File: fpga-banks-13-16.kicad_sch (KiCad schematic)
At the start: 40 parts, among them U14 XC7A100T-FGG484, U15 Oscillator_100MHz_AMJMEFB

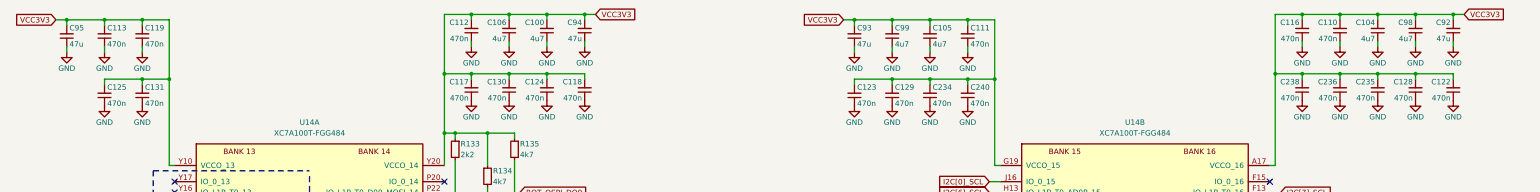
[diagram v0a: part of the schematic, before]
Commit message: [#82378] Project refresh 81589
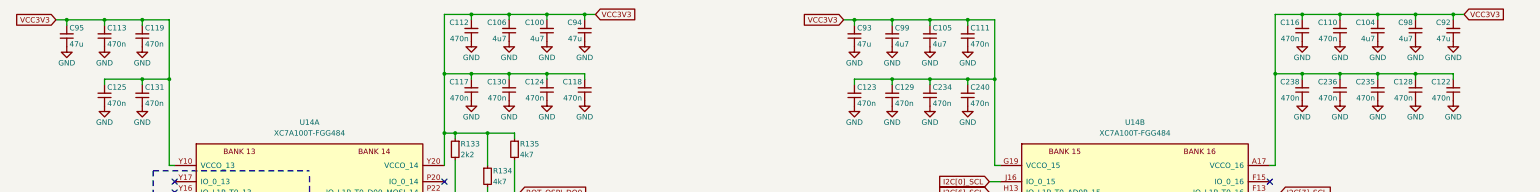
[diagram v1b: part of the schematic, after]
